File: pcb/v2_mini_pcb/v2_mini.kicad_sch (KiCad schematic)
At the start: 0 parts

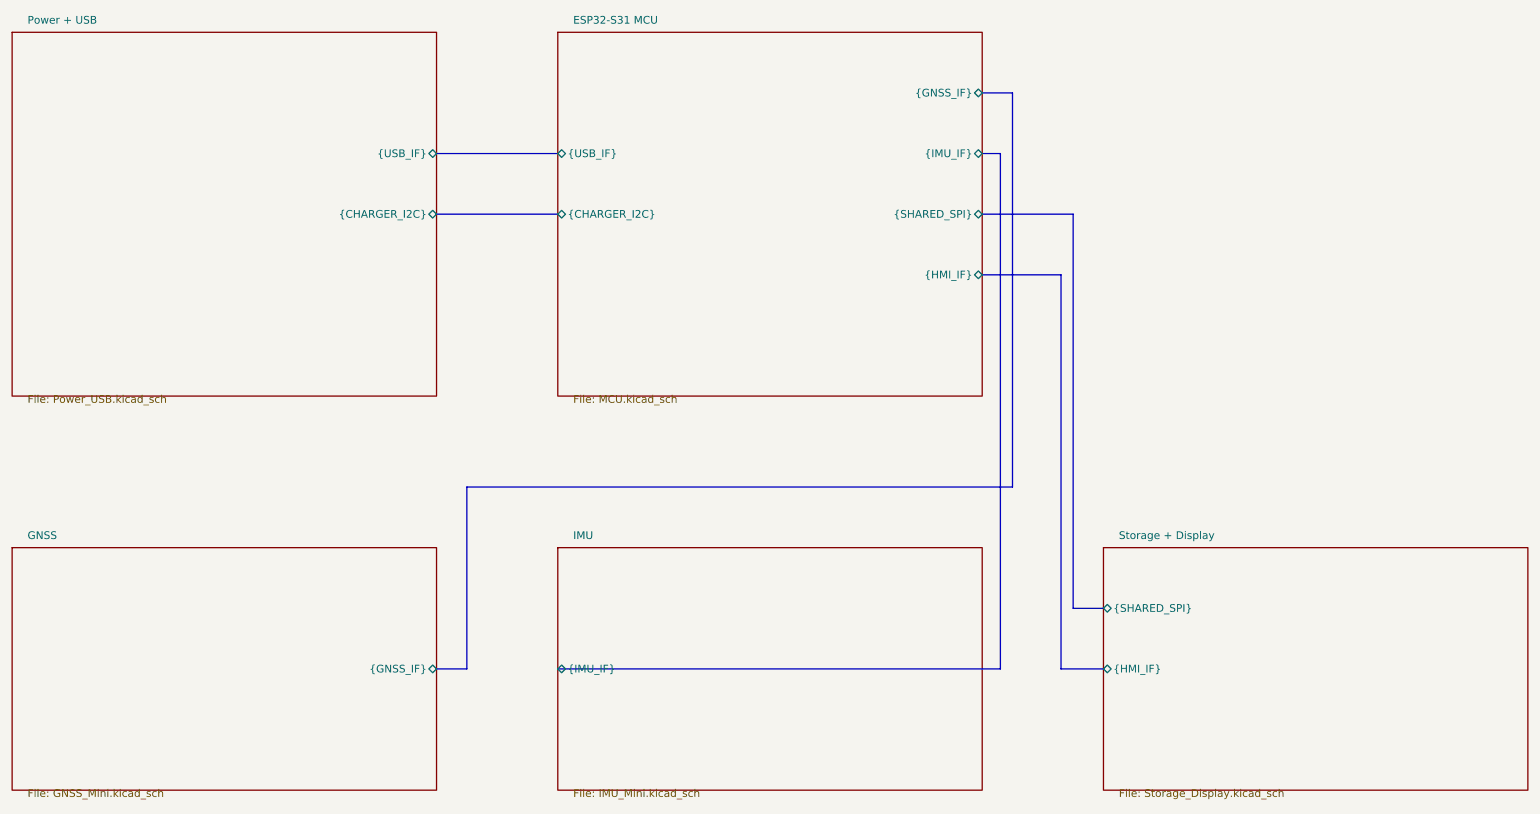
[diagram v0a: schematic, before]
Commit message: fix minor edc rules
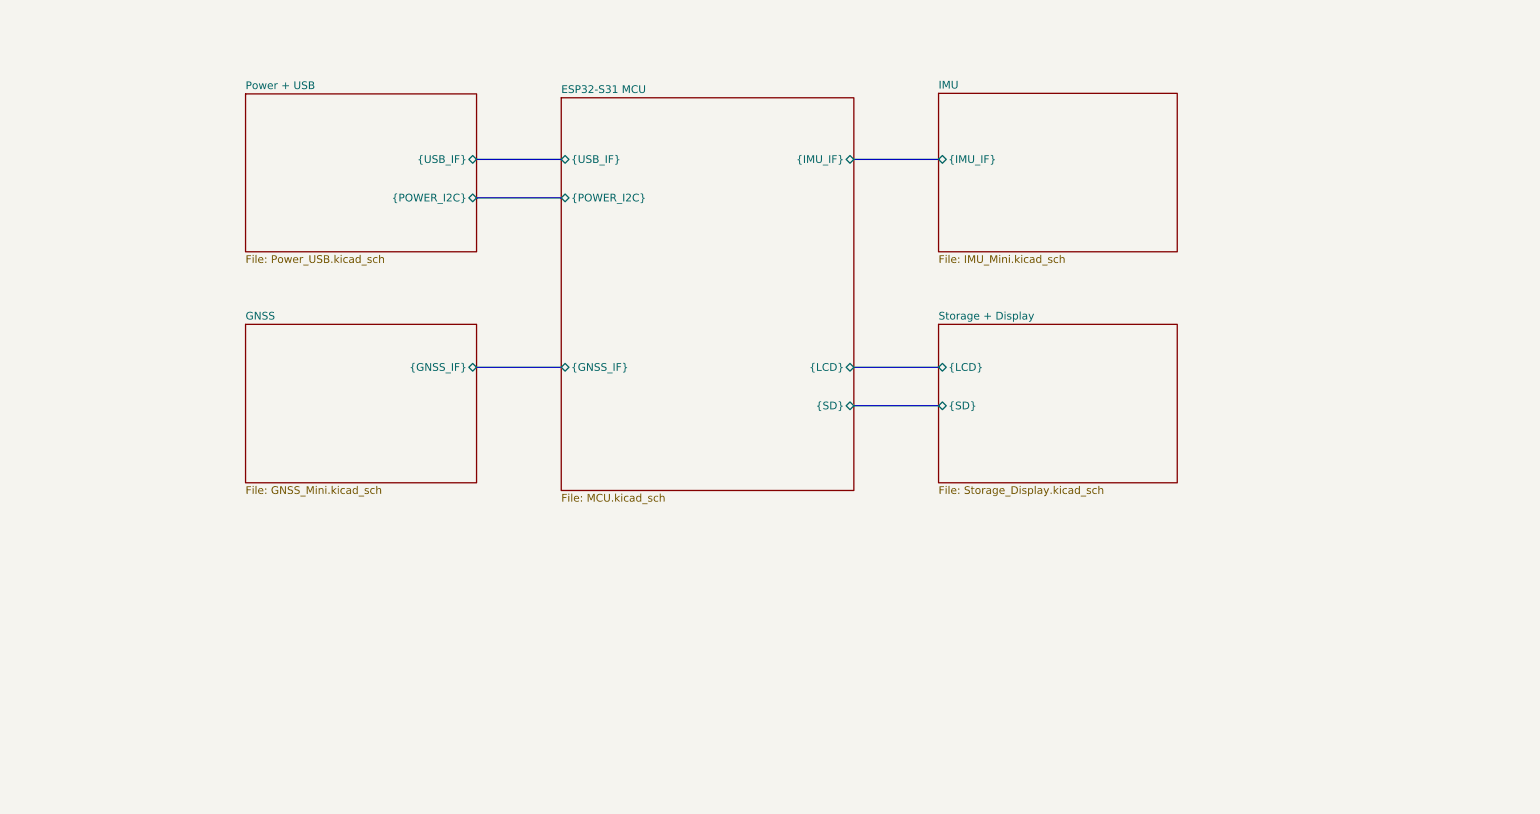
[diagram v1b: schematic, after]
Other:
- sheet ESP32-S31 MCU ports: added {LCD}, {POWER_I2C}, {SD}; removed {CHARGER_I2C}, {HMI_IF}, {SHARED_SPI}
- sheet Power + USB ports: added {POWER_I2C}; removed {CHARGER_I2C}
- sheet Storage + Display ports: added {LCD}, {SD}; removed {HMI_IF}, {SHARED_SPI}
